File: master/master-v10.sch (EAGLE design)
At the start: 43 parts, among them IC2 DS3231/SO, J1 AVR_SPI_PRG_6PTH, J2 TWIG-2.0-DIPD, J3 TWIG-2.0-DIPD, J4 TWIG-2.0-DIPD, U1 MCP9804, U2 ATMEGA640/1280/2560-A, U3 FT232RL-BASICSSOP, U4 AP1117E, U5 USD-SOCKETNEW, U6 INA169

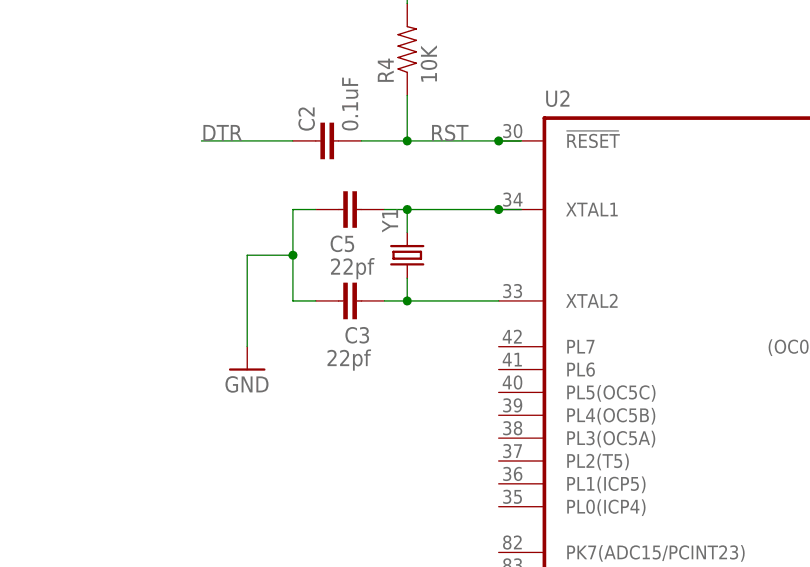
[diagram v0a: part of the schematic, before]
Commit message: add resonator
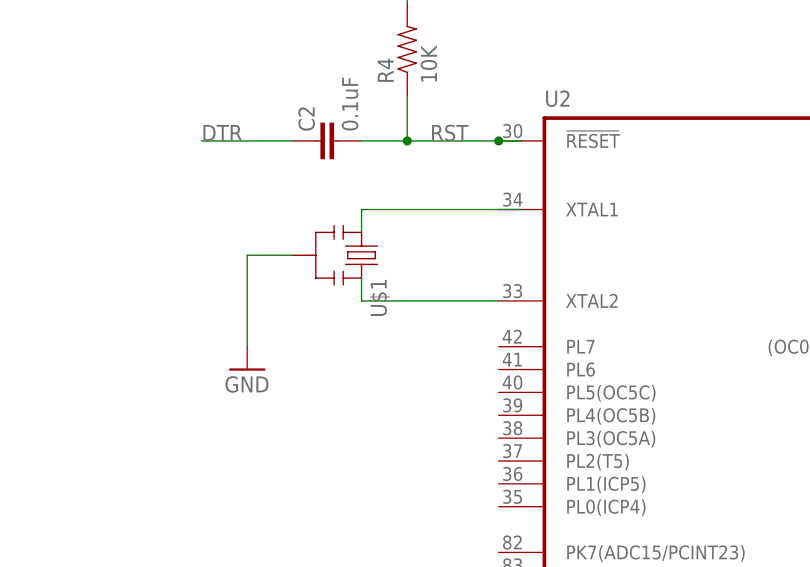
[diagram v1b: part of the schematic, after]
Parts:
- removed C3, C5: 22pf, SparkFun-Capacitors:CAP0805
- removed Y1: (no value), SparkFun-FreqCtrl:CRYSTALHC49US
- added U$1: (no value), resonador:RESONATOR-SMD
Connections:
- removed net N$21: C5.1, U2.XTAL1, Y1.2
- removed net N$22: C3.2, U2.XTAL2, Y1.1
- new net N$14: U$1.3, U2.XTAL2
- new net N$2: U$1.1
- net GND: now also U$1.2; no longer C3.1, C5.2
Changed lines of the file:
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@@
 <part name="LED1" library="adafruit" deviceset="LED" device="CHIPLED_0805"/>
 <part name="LED2" library="adafruit" deviceset="LED" device="CHIPLED_0805" value="RED"/>
-<part name="C3" library="SparkFun-Capacitors" deviceset="CAP" device="0805" value="22pf"/>
-<part name="C5" library="SparkFun-Capacitors" deviceset="CAP" device="0805" value="22pf"/>
 <part name="B1" library="battery" deviceset="CR1220" device=""/>
 <part name="C6" library="SparkFun" deviceset="CAP" device="0402-CAP" value="0.1uF"/>
@@
 <part name="FRAME1" library="SparkFun-Aesthetics" deviceset="FRAME-LEDGER" device=""/>
 <part name="U4" library="v-reg" deviceset="AP1117" device="E"/>
-<part name="Y1" library="SparkFun-FreqCtrl" deviceset="CRYSTAL" device="HC49US"/>
 <part name="GND18" library="SparkFun" deviceset="GND" device=""/>
 <part name="R10" library="SparkFun" deviceset="RESISTOR" device="0402-RES" value="10k"/>
@@
 <part name="GND16" library="SparkFun" deviceset="GND" device=""/>
 <part name="SUPPLY10" library="SparkFun-Aesthetics" deviceset="3.3V" device=""/>
+<part name="U$1" library="resonador" deviceset="RESONATOR-" device="SMD"/>
 </parts>
 <sheets>
@@
 <instance part="LED1" gate="G$1" x="266.7" y="187.96"/>
 <instance part="LED2" gate="G$1" x="160.02" y="99.06"/>
-<instance part="C3" gate="G$1" x="160.02" y="223.52" smashed="yes" rot="R90">
-<attribute name="NAME" x="161.036" y="220.599" size="1.778" layer="95" rot="R180"/>
-<attribute name="VALUE" x="161.036" y="218.059" size="1.778" layer="96" rot="R180"/>
-</instance>
-<instance part="C5" gate="G$1" x="157.48" y="233.68" smashed="yes" rot="R270">
-<attribute name="NAME" x="156.464" y="228.981" size="1.778" layer="95"/>
-<attribute name="VALUE" x="156.464" y="226.441" size="1.778" layer="96"/>
-</instance>
 <instance part="B1" gate="G$1" x="50.8" y="58.42" rot="R90"/>
 <instance part="C6" gate="G$1" x="66.04" y="58.42" smashed="yes">
@@
 <instance part="FRAME1" gate="G$2" x="330.2" y="0"/>
 <instance part="U4" gate="G$1" x="27.94" y="251.46"/>
-<instance part="Y1" gate="G$1" x="165.1" y="228.6" rot="R90"/>
 <instance part="GND18" gate="1" x="147.32" y="215.9"/>
 <instance part="R10" gate="G$1" x="292.1" y="154.94"/>
@@
 <instance part="GND16" gate="1" x="294.64" y="187.96" rot="R180"/>
 <instance part="SUPPLY10" gate="G$1" x="294.64" y="175.26" rot="R180"/>
+<instance part="U$1" gate="G$1" x="160.02" y="228.6" rot="R270"/>
 </instances>
 <busses>
@@
 </segment>
 <segment>
-<pinref part="C5" gate="G$1" pin="2"/>
-<wire x1="154.94" y1="233.68" x2="152.4" y2="233.68" width="0.1524" layer="91"/>
-<wire x1="152.4" y1="233.68" x2="152.4" y2="228.6" width="0.1524" layer="91"/>
-<pinref part="C3" gate="G$1" pin="1"/>
-<wire x1="152.4" y1="228.6" x2="152.4" y2="223.52" width="0.1524" layer="91"/>
-<wire x1="152.4" y1="223.52" x2="154.94" y2="223.52" width="0.1524" layer="91"/>
 <pinref part="GND18" gate="1" pin="GND"/>
 <wire x1="152.4" y1="228.6" x2="147.32" y2="228.6" width="0.1524" layer="91"/>
 <wire x1="147.32" y1="228.6" x2="147.32" y2="218.44" width="0.1524" layer="91"/>
-<junction x="152.4" y="228.6"/>
+<pinref part="U$1" gate="G$1" pin="2"/>
 </segment>
 <segment>
@@
 </segment>
 </net>
-<net name="N$21" class="0">
-<segment>
-<pinref part="Y1" gate="G$1" pin="2"/>
-<wire x1="177.8" y1="233.68" x2="175.26" y2="233.68" width="0.1524" layer="91"/>
-<wire x1="175.26" y1="233.68" x2="165.1" y2="233.68" width="0.1524" layer="91"/>
-<wire x1="165.1" y1="233.68" x2="165.1" y2="231.14" width="0.1524" layer="91"/>
-<pinref part="C5" gate="G$1" pin="1"/>
-<wire x1="162.56" y1="233.68" x2="165.1" y2="233.68" width="0.1524" layer="91"/>
-<junction x="165.1" y="233.68"/>
-<pinref part="U2" gate="G$1" pin="XTAL1"/>
-<junction x="175.26" y="233.68"/>
-</segment>
-</net>
-<net name="N$22" class="0">
-<segment>
-<pinref part="U2" gate="G$1" pin="XTAL2"/>
-<pinref part="Y1" gate="G$1" pin="1"/>
-<wire x1="175.26" y1="223.52" x2="165.1" y2="223.52" width="0.1524" layer="91"/>
-<wire x1="165.1" y1="223.52" x2="165.1" y2="226.06" width="0.1524" layer="91"/>
-<pinref part="C3" gate="G$1" pin="2"/>
-<wire x1="162.56" y1="223.52" x2="165.1" y2="223.52" width="0.1524" layer="91"/>
-<junction x="165.1" y="223.52"/>
-</segment>
-</net>
 <net name="CD" class="0">
 <segment>
@@
 </segment>
 </net>
+<net name="N$2" class="0">
+<segment>
+<wire x1="177.8" y1="233.68" x2="160.02" y2="233.68" width="0.1524" layer="91"/>
+<wire x1="160.02" y1="233.68" x2="160.02" y2="231.14" width="0.1524" layer="91"/>
+<pinref part="U$1" gate="G$1" pin="1"/>
+</segment>
+</net>
+<net name="N$14" class="0">
+<segment>
+<pinref part="U2" gate="G$1" pin="XTAL2"/>
+<wire x1="175.26" y1="223.52" x2="160.02" y2="223.52" width="0.1524" layer="91"/>
+<pinref part="U$1" gate="G$1" pin="3"/>
+<wire x1="160.02" y1="223.52" x2="160.02" y2="226.06" width="0.1524" layer="91"/>
+</segment>
+</net>
